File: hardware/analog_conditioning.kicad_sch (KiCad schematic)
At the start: 39 parts, among them J1 AudioJack2, J2 AudioJack2, J4 Conn_02x05_Odd_Even, U1 TL072, U2 TL072, U201 MCP6002-xSN

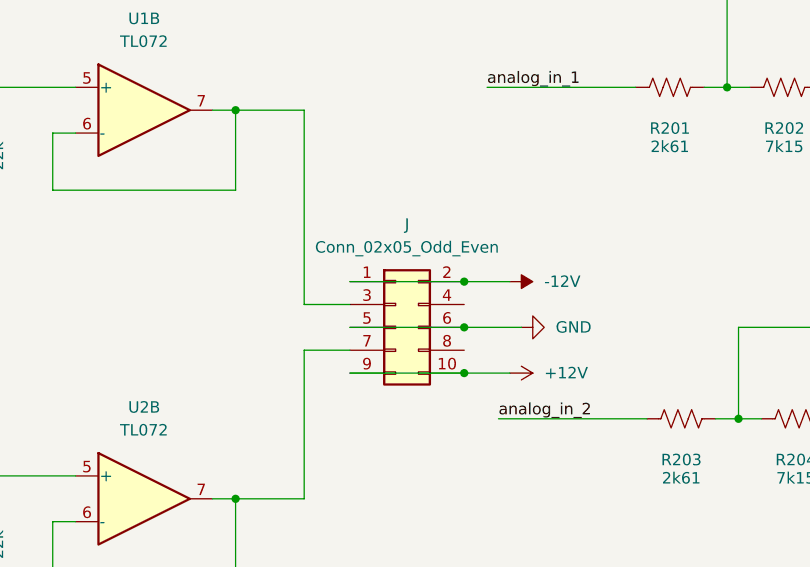
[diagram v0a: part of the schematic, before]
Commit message: hardware update
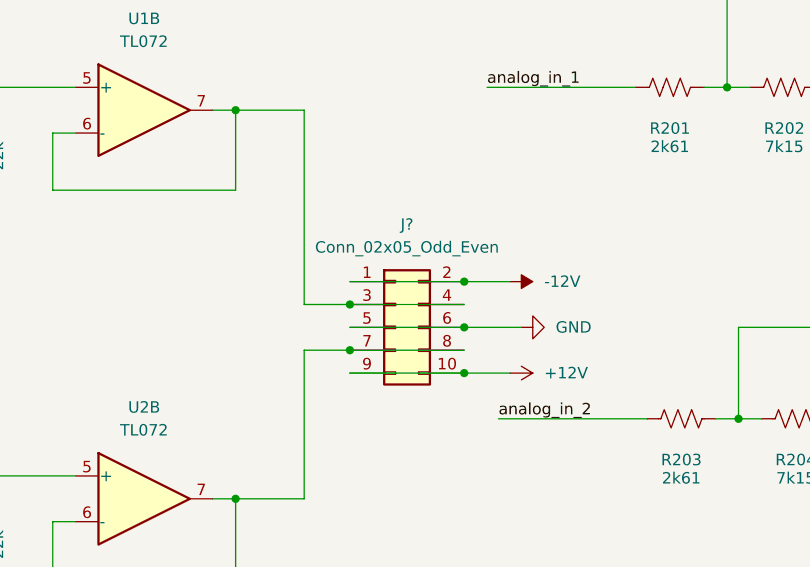
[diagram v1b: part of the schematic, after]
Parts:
- renumbered J to J?
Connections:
- net at J?.3 (Pin_3), U1.6 (-), U1.7: now also J?.4 (Pin_4)
- net at J?.7 (Pin_7), U2.6 (-), U2.7: now also J?.8 (Pin_8)
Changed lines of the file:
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@@
 	)
 	(junction
+		(at 172.72 68.58)
+		(diameter 0)
+		(color 0 0 0 0)
+	)
+	(junction
+		(at 172.72 63.5)
+		(diameter 0)
+		(color 0 0 0 0)
+	)
+	(junction
 		(at 228.6 76.2)
 		(diameter 0)
@@
 	(wire
 		(pts
+			(xy 172.72 68.58) (xy 185.42 68.58)
+		)
+		(stroke
+			(width 0)
+			(type default)
+		)
+	)
+	(wire
+		(pts
 			(xy 91.44 123.19) (xy 80.01 123.19)
 		)
@@
 	(wire
 		(pts
+			(xy 172.72 63.5) (xy 185.42 63.5)
+		)
+		(stroke
+			(width 0)
+			(type default)
+		)
+	)
+	(wire
+		(pts
 			(xy 114.3 82.55) (xy 115.57 82.55)
 		)
@@
 		(dnp no)
 		(fields_autoplaced yes)
-		(property "Reference" "#PWR"
+		(property "Reference" "#PWR?"
 			(at 57.15 147.32 0)
 			(effects
@@
 		(pin "1"
 		)
-		(instances)
+		(instances
+			(project "dmx_controller"
+				(path "/c888dd99-01b7-4b4b-82e5-501bcedd41ed/05e4dc0b-bade-45d2-8fa1-6b1ecf425979"
+					(reference "#PWR?")
+					(unit 1)
+				)
+			)
+		)
 	)
 	(symbol
@@
 		(dnp no)
 		(fields_autoplaced yes)
-		(property "Reference" "J"
+		(property "Reference" "J?"
 			(at 179.07 54.61 0)
 			(effects
@@
 		(pin "8"
 		)
-		(instances)
+		(instances
+			(project "dmx_controller"
+				(path "/c888dd99-01b7-4b4b-82e5-501bcedd41ed/05e4dc0b-bade-45d2-8fa1-6b1ecf425979"
+					(reference "J?")
+					(unit 1)
+				)
+			)
+		)
 	)
 	(symbol
@@
 		(dnp no)
 		(fields_autoplaced yes)
-		(property "Reference" "#PWR"
+		(property "Reference" "#PWR?"
 			(at 57.15 124.46 0)
 			(effects
@@
 		(pin "1"
 		)
-		(instances)
+		(instances
+			(project "dmx_controller"
+				(path "/c888dd99-01b7-4b4b-82e5-501bcedd41ed/05e4dc0b-bade-45d2-8fa1-6b1ecf425979"
+					(reference "#PWR?")
+					(unit 1)
+				)
+			)
+		)
 	)
 )

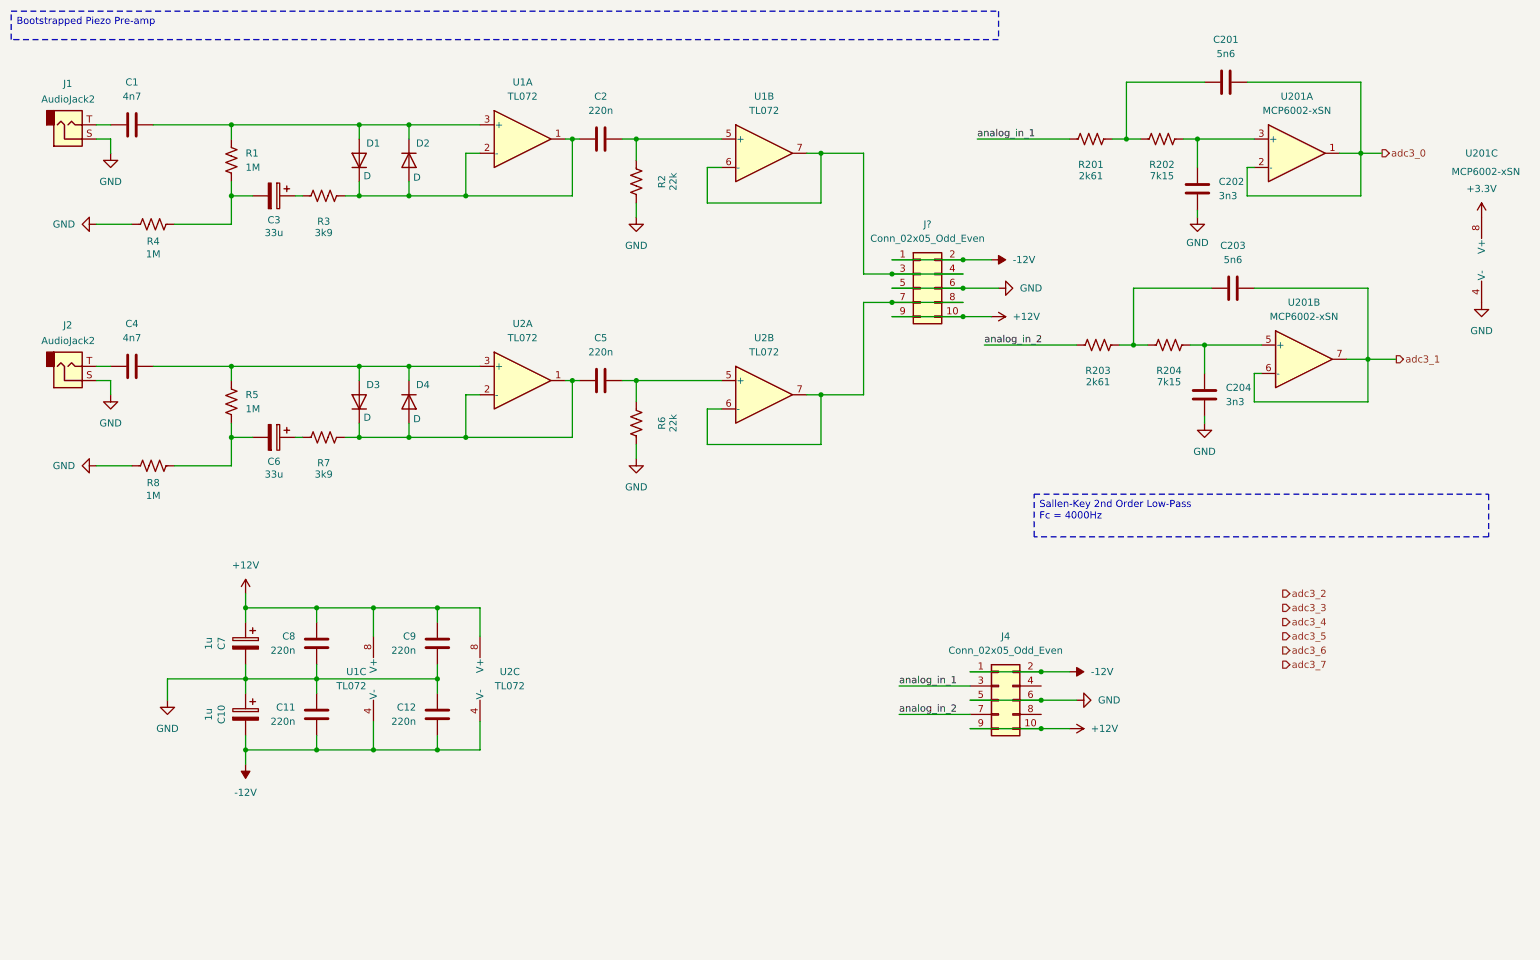
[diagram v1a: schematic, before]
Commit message: hardware update
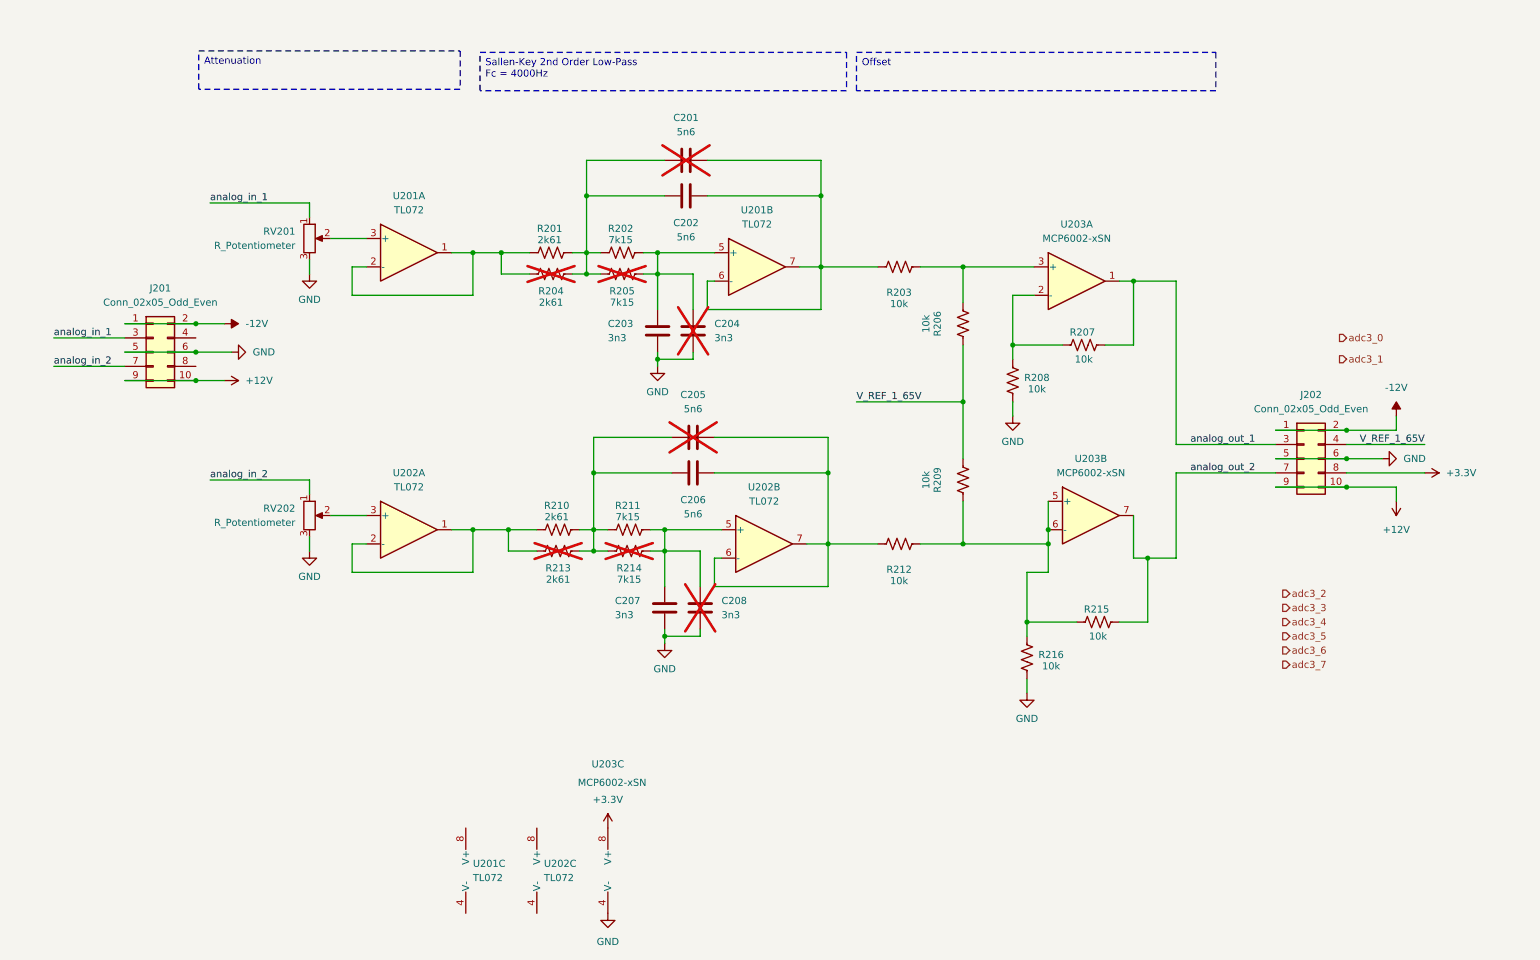
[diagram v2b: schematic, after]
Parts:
- removed C1, C4: 4n7, Capacitor_SMD:C_0805_2012Metric, symbol Device:C
- removed C10, C7: 1u, Capacitor_SMD:CP_Elec_4x5.4, symbol Device:C_Polarized
- removed C11, C12, C2, C5, C8, C9: 220n, Capacitor_SMD:C_0805_2012Metric, symbol Device:C
- removed C203: 5n6, Capacitor_SMD:C_0805_2012Metric, symbol Device:C
- removed C3, C6: 33u, Capacitor_SMD:CP_Elec_6.3x5.8, symbol Device:C_Polarized
- removed D1, D2, D3, D4: D, Diode_SMD:D_SOD-323_HandSoldering, symbol Device:D
- removed J1, J2: AudioJack2, Connector_Audio:Jack_6.35mm_Neutrik_NMJ6HFD2-AU_Horizontal, symbol Connector_Audio:AudioJack2
- removed J?: Conn_02x05_Odd_Even, Connector_IDC:IDC-Header_2x05_P2.54mm_Vertical, symbol Connector_Generic:Conn_02x05_Odd_Even
- removed R1, R4, R5, R8: 1M, Resistor_SMD:R_0805_2012Metric, symbol Device:R_US
- removed R2, R6: 22k, Resistor_SMD:R_0805_2012Metric, symbol Device:R_US
- removed R3, R7: 3k9, Resistor_SMD:R_0805_2012Metric, symbol Device:R_US
- removed U1, U2: TL072, Package_SO:SOIC-8_3.9x4.9mm_P1.27mm, symbol Amplifier_Operational:TL072
- added C201, C205, C206: 5n6, Capacitor_SMD:C_0805_2012Metric, symbol Device:C
- added C207, C208: 3n3, Capacitor_SMD:C_0805_2012Metric, symbol Device:C
- added J202: Conn_02x05_Odd_Even, Connector_IDC:IDC-Header_2x05_P2.54mm_Vertical, symbol Connector_Generic:Conn_02x05_Odd_Even
- added R205, R211, R214: 7k15, Resistor_SMD:R_0805_2012Metric, symbol Device:R_US
- added R206, R207, R208, R209, R212, R215, R216: 10k, Resistor_SMD:R_0805_2012Metric, symbol Device:R_US
- added R210, R213: 2k61, Resistor_SMD:R_0805_2012Metric, symbol Device:R_US
- added RV201, RV202: R_Potentiometer, symbol Device:R_Potentiometer
- added U201, U202: TL072, Package_SO:SOIC-8_3.9x4.9mm_P1.27mm, symbol Amplifier_Operational:TL072
- C204: now not fitted
- R203: value 2k61 -> 10k
- R204: value 7k15 -> 2k61; now not fitted
- renumbered C201 to C202, C202 to C203, J4 to J201, U201 to U203
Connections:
- net +12V: now also J202.10 (Pin_10), J202.9 (Pin_9)
- net +3.3V: now also J202.8 (Pin_8)
- net -12V: now also J202.1 (Pin_1), J202.2 (Pin_2)
- net GND: now also C207.2, C208.2, J202.5 (Pin_5), J202.6 (Pin_6), R208.2, R216.2, RV201.3, RV202.3
- net adc3_0: no longer C202.2, U203.1, U203.2 (-)
- net adc3_1: no longer U203.6 (-), U203.7
- net analog_in_1: now also RV201.1; no longer R201.1
- net analog_in_2: now also RV202.1; no longer R203.1
- net at R203.2: now also U203.3 (+), R206.1; no longer R204.1
- net at C203.1, R202.2: now also C204.1, R205.2, U201.5 (+); no longer U203.3 (+)
- net at C202.1, R201.2, R202.1: now also R204.2, C201.1, R205.1
- new net: R209.2, R212.2, R215.2, R216.1, U203.5 (+), U203.6 (-)
- new net: C205.1, C206.1, R210.2, R211.1, R213.2, R214.1
- new net: C207.1, C208.1, R211.2, R214.2, U202.5 (+)
- new net: C205.2, C206.2, R212.1, U202.6 (-), U202.7
- new net: C201.2, C202.2, R203.1, U201.6 (-), U201.7
- new net: R210.1, R213.1, U202.1, U202.2 (-)
- new net: RV202.2, U202.3 (+)
- new net: R207.2, R208.1, U203.2 (-)
- new net: R201.1, R204.1, U201.1, U201.2 (-)
- new net: RV201.2, U201.3 (+)
- new net V_REF_1_65V: J202.4 (Pin_4), R206.2, R209.1
- new net analog_out_1: J202.3 (Pin_3), R207.1, U203.1
- new net analog_out_2: J202.7 (Pin_7), R215.1, U203.7
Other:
- moved on the sheet: C202, C203, J201, R201, R202, U203A, U203B, U203C
